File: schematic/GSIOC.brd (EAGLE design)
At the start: 30 x 60 mm, 39 parts, among them Q1 IRLML5203, X2 PN61729-S, X3 22-23-2081, X6 22-23-2091

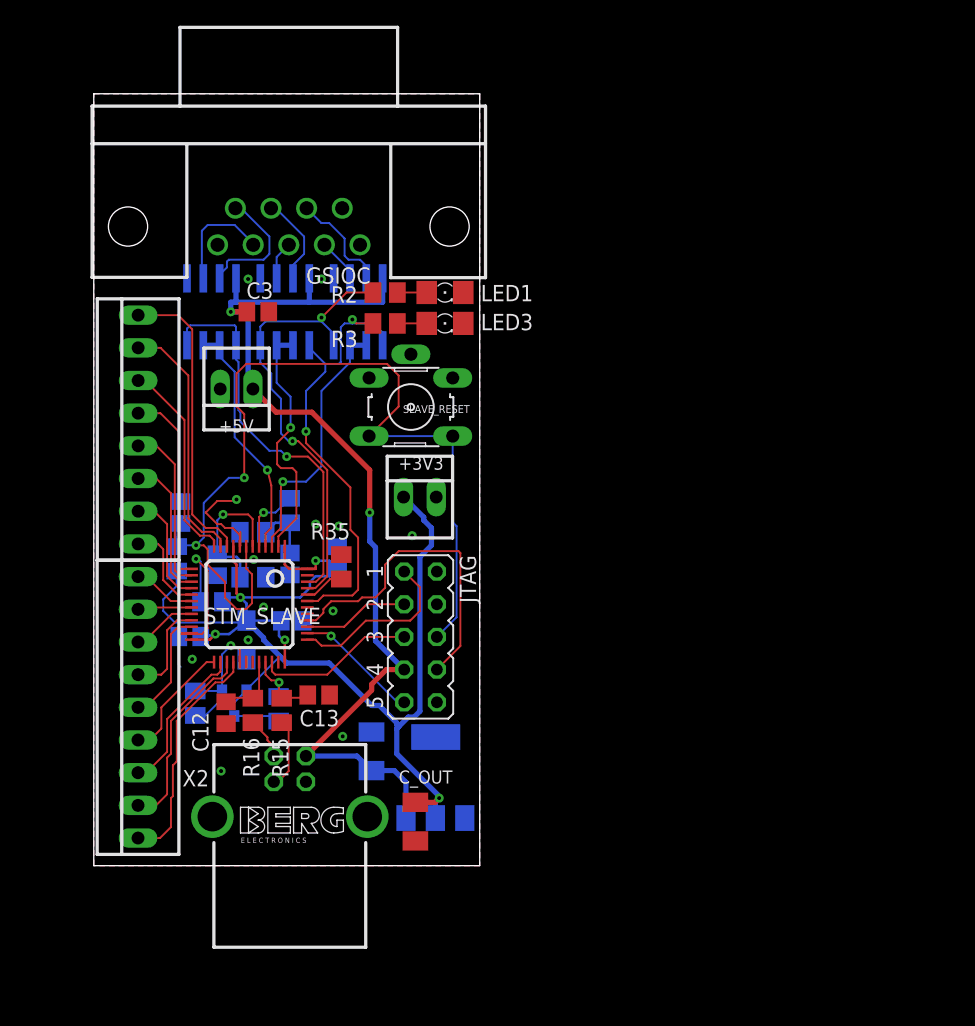
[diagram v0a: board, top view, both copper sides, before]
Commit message: cd /home/dekar/eagle/peptidatorV0.51
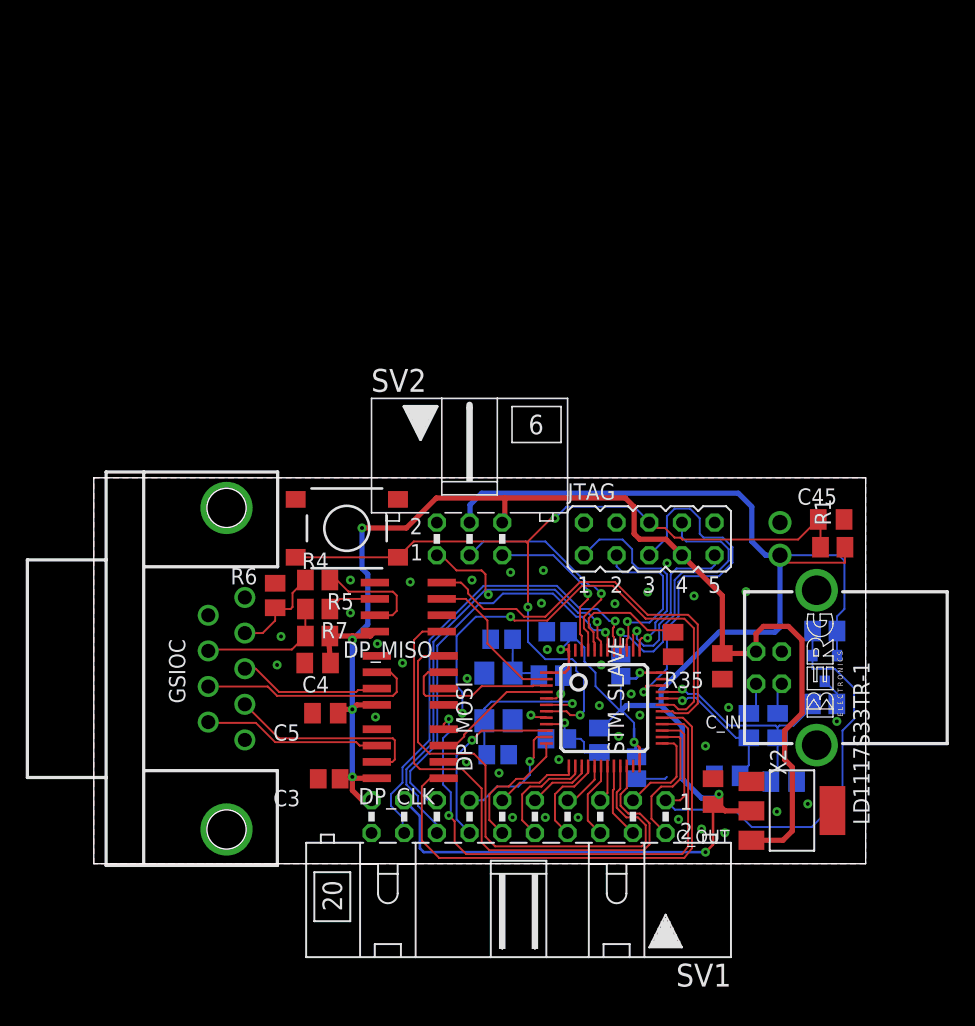
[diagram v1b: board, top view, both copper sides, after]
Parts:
- removed +3V3, +5V: 22-23-2021, con-molex:22-23-2021
- removed C36: 10u, resistor:SMC_A
- removed LED1, LED3: (no value), led:1206
- removed R2, R3: 220, resistor:M0805
- removed SLAVE_RESET: 10-XXG, switch-omron:B3F-10XXG
- removed X3: 22-23-2081, con-molex:22-23-2081
- removed X6: 22-23-2091, con-molex:22-23-2091
- added C4, C5: 100n, rcl:C0805K
- added L1: SPECIAL, resistor:M0805
- added R4, R5: 220, resistor:M0805
- added R6, R7: 1k, resistor:M0805
- added S1: DTSM-6, switch-tact:DTSM-6
- added SV1: (no value), con-harting-ml:ML20L
- added SV2: (no value), con-ml:ML6L
- C12, C13, C45: device resistor:C0805 -> rcl:C0805K
- C_IN, C_OUT: device rcl:C1206K -> rcl:C0805K
- QF2: device crystal:ACT530SMX -> smdQuartz:ACT_530SMX
- moved R1 51.0 mm to (57.4, 24.8), flipped to the top, turned to 180 degrees
- moved C45 50.6 mm to (57.3, 26.9), flipped to the top, turned to 0 degrees
- moved R14 49.3 mm to (56.8, 18.2), turned to 180 degrees
- moved Q1 46.0 mm to (56.8, 15.3)
- moved X2 42.6 mm to (56.2, 15.4), turned to 90 degrees
- moved R32 42.4 mm to (56.8, 12.6), turned to 0 degrees
- moved C12 39.3 mm to (49.2, 6.99), flipped to the bottom, turned to 0 degrees
- moved R15 38.6 mm to (53.2, 10.9), flipped to the bottom, turned to 270 degrees
- moved R16 38.6 mm to (50.9, 10.9), flipped to the bottom, turned to 270 degrees
- moved DP_CLK 37.7 mm to (24.6, 8.70), flipped to the top, turned to 90 degrees
- moved C13 36.8 mm to (53.6, 6.54), flipped to the bottom, turned to 180 degrees
- moved C3 36.7 mm to (18.3, 6.75), turned to 180 degrees
- moved C31 36.2 mm to (42.2, 7.61), turned to 270 degrees
- moved GSIOC 34.7 mm to (10.3, 15.3), turned to 270 degrees
- moved DP_MOSI 30.3 mm to (24.6, 14.4), flipped to the top, turned to 90 degrees
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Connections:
- net N$28 renamed OSC<=
- net N$34 renamed OSC=>
- removed net CLK: DP_CLK.1, DP_CLK.4, STM_SLAVE.46
- removed net N$2: LED3.A, R3.1
- removed net N$4: STM_SLAVE.22, X6.5
- removed net USART1_RX: DP_MISO.1, DP_MOSI.1, R3.2, STM_SLAVE.43
- removed net USART1_TX: DP_MISO.4, DP_MOSI.4, R2.2, STM_SLAVE.45
- new net N$3: GSIOC.2, R4.2, R6.1
- new net N$5: GSIOC.7, R5.2, R7.2
- new net PA10: DP_MOSI.1, STM_SLAVE.31
- new net PA9: DP_MISO.4, STM_SLAVE.30
- new net PB11: DP_MISO.1, STM_SLAVE.22
- new net PB5: STM_SLAVE.41, SV1.18
- new net PB6: STM_SLAVE.42, SV1.15
- new net PB7: STM_SLAVE.43, SV1.16, SV2.1
- new net PB8: STM_SLAVE.45, SV2.3
- new net PB9: STM_SLAVE.46, SV2.5
- net +5V: now also C4.1, C5.1, R7.1, SV1.19, SV2.6; no longer +5V.1
- net CLK_A: now also GSIOC.9; no longer GSIOC.4
- net CLK_B: now also GSIOC.4; no longer GSIOC.9
- net GND: now also C4.2, C5.2, DP_CLK.2, DP_MISO.2, DP_MOSI.2, GSIOC.5, R6.2, S1.3, S1.4, SV1.20, SV2.2, X2.S1, X2.S2; no longer +3V3.2, +5V.2, C36.-, LED1.C, LED3.C, SLAVE_RESET.1, SLAVE_RESET.2, SLAVE_RESET.G, X2.SHLD@1, X2.SHLD@2
- net MISO_A: now also R5.1; no longer GSIOC.2
- net MISO_B: now also R4.1; no longer GSIOC.7
- net MOSI_A: now also GSIOC.8; no longer GSIOC.3
- net MOSI_B: now also GSIOC.3; no longer GSIOC.8
- net N$1: now also C11.1, L1.2, STM_SLAVE.9; no longer LED1.A, R2.1
- net PA0: now also SV1.14; no longer X3.8
- net PA1: now also SV1.13; no longer X3.7
- net PA2: now also SV1.12; no longer X3.6
- net PA3: now also SV1.11; no longer X3.5
- net PA4: now also SV1.10; no longer X3.4
- net PA5: now also SV1.9; no longer X3.3
- net PA6: now also SV1.8; no longer X3.2
- net PA7: now also SV1.7; no longer X3.1
- net PA8: now also DP_CLK.1; no longer Q1.1, R14.1
- net PB0: now also SV1.6; no longer X6.9
- net PB1: now also SV1.5; no longer X6.8
- net PB10: now also DP_MOSI.4; no longer X6.6
- net PB12: now also SV1.3; no longer X6.4
- net PB13: now also SV1.2; no longer X6.3
- net PB14: now also Q1.1, R14.1, SV1.1; no longer X6.2
- net PB15: now also DP_CLK.4; no longer X6.1
- net PB2: now also SV1.4; no longer X6.7
- net PC13: now also DP_MISO.3; no longer DP_MOSI.2, DP_MOSI.3
- net PC14: now also DP_MOSI.3; no longer DP_MISO.2, DP_MISO.3
- net PC15: no longer DP_CLK.2
- net RESET: now also S1.1, S1.2; no longer SLAVE_RESET.3, SLAVE_RESET.4
- net VCC: now also L1.1, SV1.17, SV2.4; no longer +3V3.1, C11.1, C36.+, STM_SLAVE.9
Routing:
- net PB11: track 0.00 -> 43.5 mm
- net VCC: track 100.2 -> 142.9 mm, vias 5 -> 6
- net PB7: track 0.00 -> 41.0 mm, vias 0 -> 2
- net PA10: track 0.00 -> 38.1 mm, vias 0 -> 2
- net USART1_RX: track 36.8 -> 0.00 mm, vias 2 -> 0
- net PB5: track 0.00 -> 36.6 mm, vias 0 -> 1
- net USART1_TX: track 36.2 -> 0.00 mm, vias 2 -> 0
- net PA9: track 0.00 -> 33.0 mm
- net PB10: track 7.67 -> 40.4 mm
- net PA8: track 7.70 -> 40.1 mm, vias 1 -> 0
- net PB6: track 0.00 -> 31.9 mm, vias 0 -> 1
- net CLK: track 30.3 -> 0.00 mm, vias 1 -> 0
- net +5V: track 77.5 -> 102.8 mm, vias 2 -> 4
- net PB14: track 15.2 -> 39.4 mm
- net PB15: track 18.1 -> 41.4 mm, vias 0 -> 2
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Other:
- board size 30 x 60 mm -> 60 x 30 mm
